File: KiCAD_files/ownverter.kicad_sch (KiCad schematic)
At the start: 10 parts, among them J101 Harting-15 and Wago 6

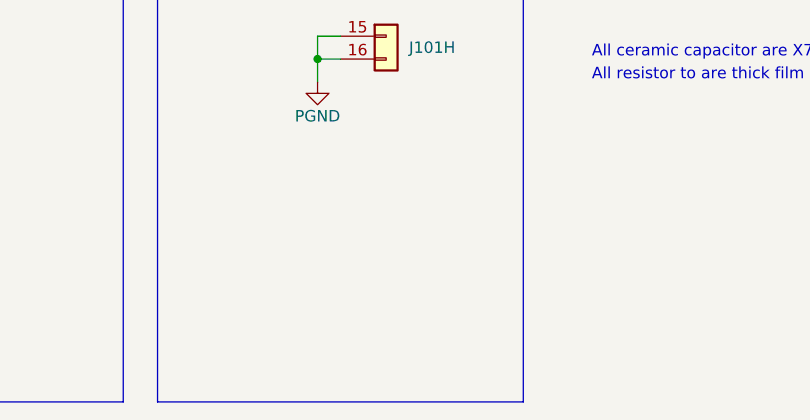
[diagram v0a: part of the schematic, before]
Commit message: wip
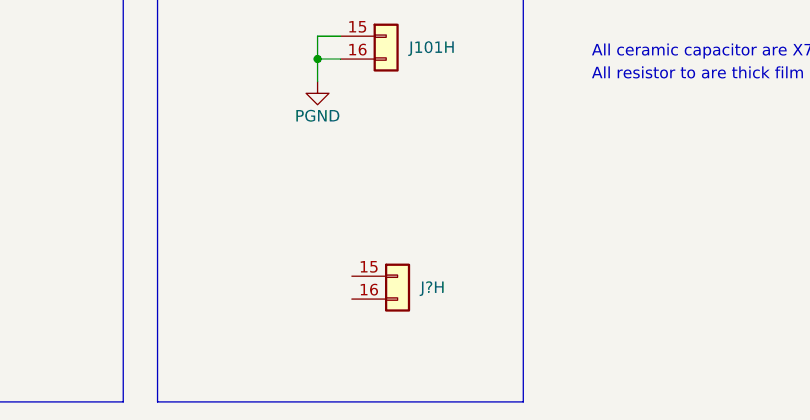
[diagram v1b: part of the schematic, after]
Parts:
- added J?: Harting-15 and Wago 6, Footprints:Harting - 15contacts and Wago, symbol Symbols:Harting 15 contacts and WAGO
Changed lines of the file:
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@@
+    )
+  )
+  (symbol (lib_id "Symbols:Harting 15 contacts and WAGO") (at 279.4 191.77 0) (unit 8)
+    (in_bom yes) (on_board yes) (dnp no) (fields_autoplaced)
+    (property "Reference" "J?" (at 281.94 193.04 0)
+      (effects (font (size 1.27 1.27)) (justify left))
+    )
+    (property "Value" "Harting-15 and Wago 6" (at 278.13 196.85 0)
+      (effects (font (size 1.27 1.27)) hide)
+    )
+    (property "Footprint" "Footprints:Harting - 15contacts and Wago" (at 278.13 186.69 0)
+      (effects (font (size 1.27 1.27)) hide)
+    )
+    (property "Datasheet" "~" (at 279.4 191.77 0)
+      (effects (font (size 1.27 1.27)) hide)
+    )
+    (property "manf#" "2604-1108" (at 279.4 191.77 0)
+      (effects (font (size 1.27 1.27)) hide)
+    )
+    (pin "1")
+    (pin "2")
+    (pin "3")
+    (pin "4")
+    (pin "5")
+    (pin "6")
+    (pin "7")
+    (pin "8")
+    (pin "10")
+    (pin "9")
+    (pin "11")
+    (pin "12")
+    (pin "13")
+    (pin "14")
+    (pin "15")
+    (pin "16")
+    (instances
+      (project "ownverter"
+        (path "/8d0c1d66-35ef-4a53-a28f-436a11b54f42"
+          (reference "J?") (unit 8)
+        )
+      )
     )
   )

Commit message: revert previous commit
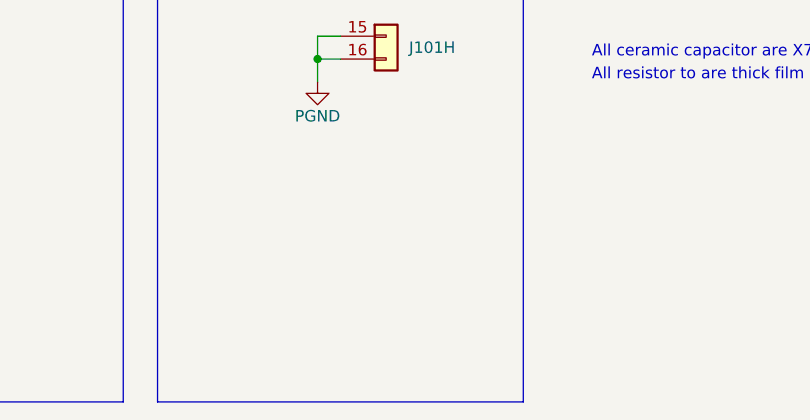
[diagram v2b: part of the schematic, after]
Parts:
- removed J?: Harting-15 and Wago 6, Footprints:Harting - 15contacts and Wago, symbol Symbols:Harting 15 contacts and WAGO
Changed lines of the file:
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@@
-    )
-  )
-  (symbol (lib_id "Symbols:Harting 15 contacts and WAGO") (at 279.4 191.77 0) (unit 8)
-    (in_bom yes) (on_board yes) (dnp no) (fields_autoplaced)
-    (property "Reference" "J?" (at 281.94 193.04 0)
-      (effects (font (size 1.27 1.27)) (justify left))
-    )
-    (property "Value" "Harting-15 and Wago 6" (at 278.13 196.85 0)
-      (effects (font (size 1.27 1.27)) hide)
-    )
-    (property "Footprint" "Footprints:Harting - 15contacts and Wago" (at 278.13 186.69 0)
-      (effects (font (size 1.27 1.27)) hide)
-    )
-    (property "Datasheet" "~" (at 279.4 191.77 0)
-      (effects (font (size 1.27 1.27)) hide)
-    )
-    (property "manf#" "2604-1108" (at 279.4 191.77 0)
-      (effects (font (size 1.27 1.27)) hide)
-    )
-    (pin "1")
-    (pin "2")
-    (pin "3")
-    (pin "4")
-    (pin "5")
-    (pin "6")
-    (pin "7")
-    (pin "8")
-    (pin "10")
-    (pin "9")
-    (pin "11")
-    (pin "12")
-    (pin "13")
-    (pin "14")
-    (pin "15")
-    (pin "16")
-    (instances
-      (project "ownverter"
-        (path "/8d0c1d66-35ef-4a53-a28f-436a11b54f42"
-          (reference "J?") (unit 8)
-        )
-      )
     )
   )
